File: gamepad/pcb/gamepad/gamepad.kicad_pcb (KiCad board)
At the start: 2 copper layers, 67.8 x 67.8 mm, 9 parts, among them U3 RP2040-ZERO

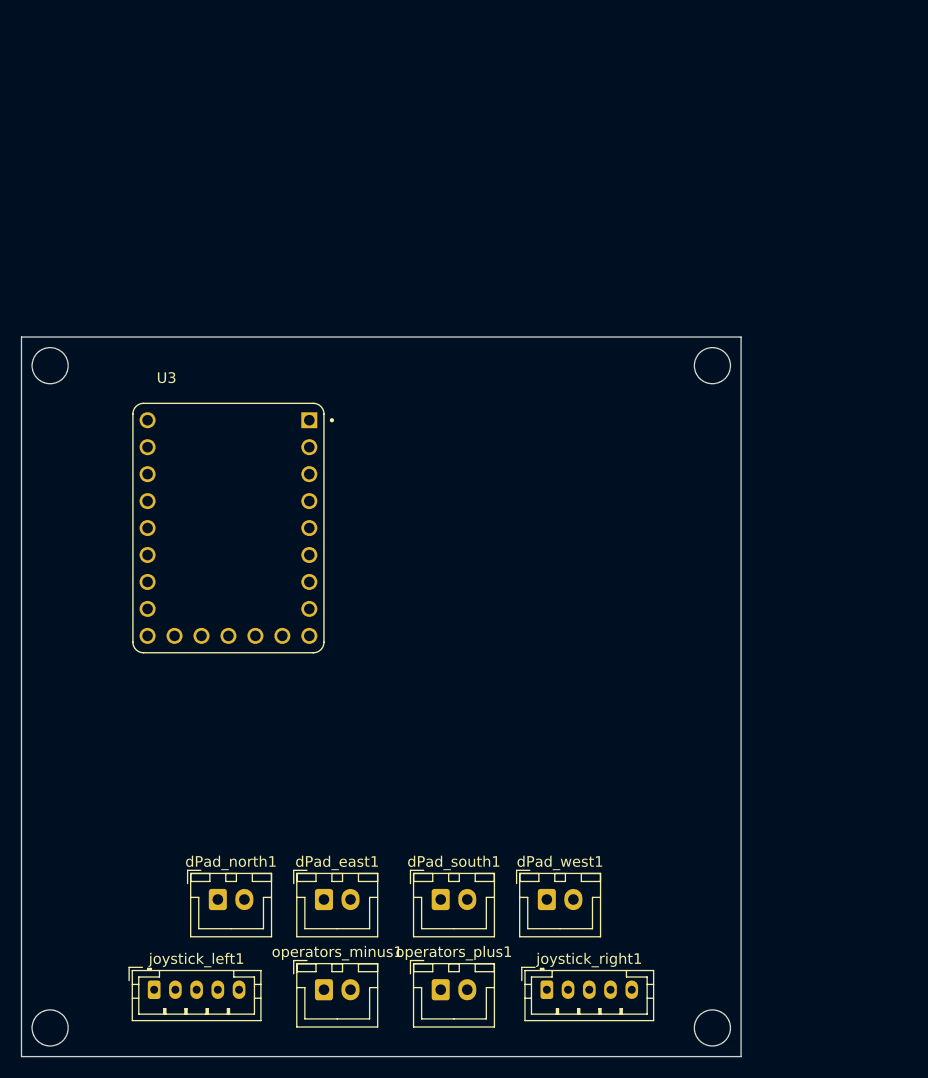
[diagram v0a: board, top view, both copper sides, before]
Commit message: upt: pcb
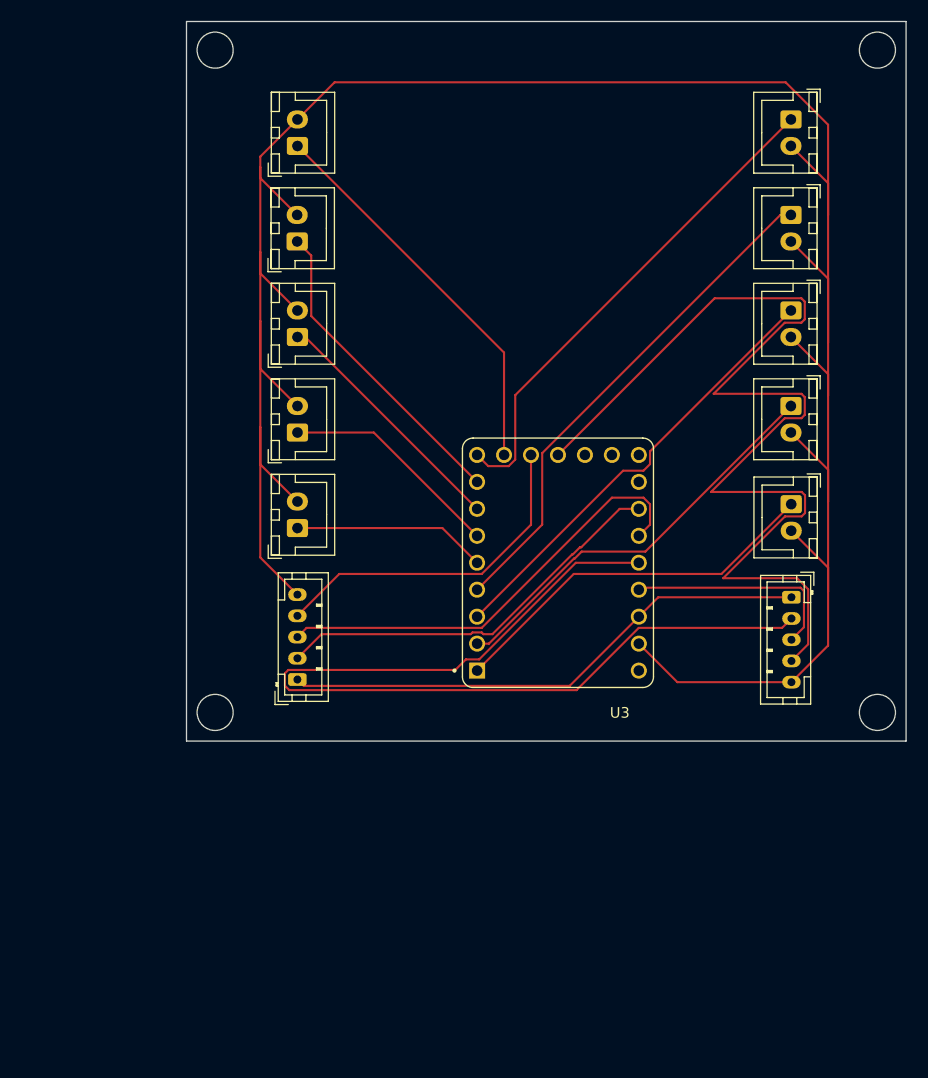
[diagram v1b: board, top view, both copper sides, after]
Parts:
- added cardinal_down1: Conn_01x02, Connector_JST:JST_XH_B2B-XH-A_1x02_P2.50mm_Vertical, F.Cu at (81.0, 55.0)
- added cardinal_left1: Conn_01x02, Connector_JST:JST_XH_B2B-XH-A_1x02_P2.50mm_Vertical, F.Cu at (81.0, 46.0)
- added cardinal_right1: Conn_01x02, Connector_JST:JST_XH_B2B-XH-A_1x02_P2.50mm_Vertical, F.Cu at (81.0, 64.0)
- added cardinal_up1: Conn_01x02, Connector_JST:JST_XH_B2B-XH-A_1x02_P2.50mm_Vertical, F.Cu at (81.0, 73.0)
- moved operators_plus1 88.4 mm to (127.5, 34.5), turned to -90 degrees
- moved operators_minus1 79.5 mm to (81.0, 37.0), turned to 90 degrees
- moved dPad_west1 68.5 mm to (127.5, 43.5), turned to -90 degrees
- moved dPad_north1 65.6 mm to (127.5, 70.8), turned to -90 degrees
- moved dPad_south1 64.6 mm to (127.5, 52.5), turned to -90 degrees
- moved dPad_east1 64.0 mm to (127.5, 61.5), turned to -90 degrees
- moved joystick_right1 43.6 mm to (127.5, 79.5), turned to -90 degrees
- moved joystick_left1 32.2 mm to (81.0, 87.3), turned to 90 degrees
- moved U3 31.2 mm to (105.5, 76.3), turned to 180 degrees
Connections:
- U3 pad 10: unconnected-(U3-GP9-Pad10) -> Net-(U3-GP9)
- U3 pad 11: unconnected-(U3-GP10-Pad11) -> Net-(U3-GP10)
- U3 pad 12: unconnected-(U3-GP11-Pad12) -> Net-(U3-GP11)
- U3 pad 9: unconnected-(U3-GP8-Pad9) -> Net-(U3-GP8)
- joystick_left1 pad 4: Net-(U3-GP6) -> Net-(U3-GP10)
- joystick_right1 pad 4: Net-(U3-GP7) -> Net-(U3-GP11)
- operators_minus1 pad 1: Net-(U3-GP5) -> Net-(U3-GP9)
- operators_plus1 pad 1: Net-(U3-GP4) -> Net-(U3-GP8)
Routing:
- net GND: track 0.00 -> 242.4 mm
- net Net-(U3-GP11): track 0.00 -> 101.6 mm
- net Net-(U3-GP28): track 0.00 -> 89.5 mm
- net +3V3: track 0.00 -> 50.3 mm
- net Net-(U3-GP3): track 0.00 -> 48.1 mm
- net Net-(U3-GP8): track 0.00 -> 47.1 mm
- net Net-(U3-GP27): track 0.00 -> 42.3 mm
- net Net-(U3-GP2): track 0.00 -> 42.2 mm
- net Net-(U3-GP1): track 0.00 -> 38.8 mm
- net Net-(U3-GP26): track 0.00 -> 38.1 mm
- net Net-(U3-GP9): track 0.00 -> 37.2 mm
- net Net-(U3-GP0): track 0.00 -> 36.1 mm
- net Net-(U3-GP10): track 0.00 -> 32.1 mm
- net Net-(U3-GP7): track 0.00 -> 29.7 mm
- net Net-(U3-GP6): track 0.00 -> 23.6 mm
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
